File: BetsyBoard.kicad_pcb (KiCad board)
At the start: 2 copper layers, 50 x 50 mm, 44 parts, among them CON1 SDMMC_Card, P1 USB_OTG, P2 Analog, P3 Digital, P4 JLINK-SWD, P5 POWER, P6 CORTEX-JTAG, SW1 SW_PUSH, U1 STM32L486Rx-LQFP64, U2 TPS63051, U3 APX823, U4 PUSBM5V5X4, X1 XTAL, Y1 Crystal

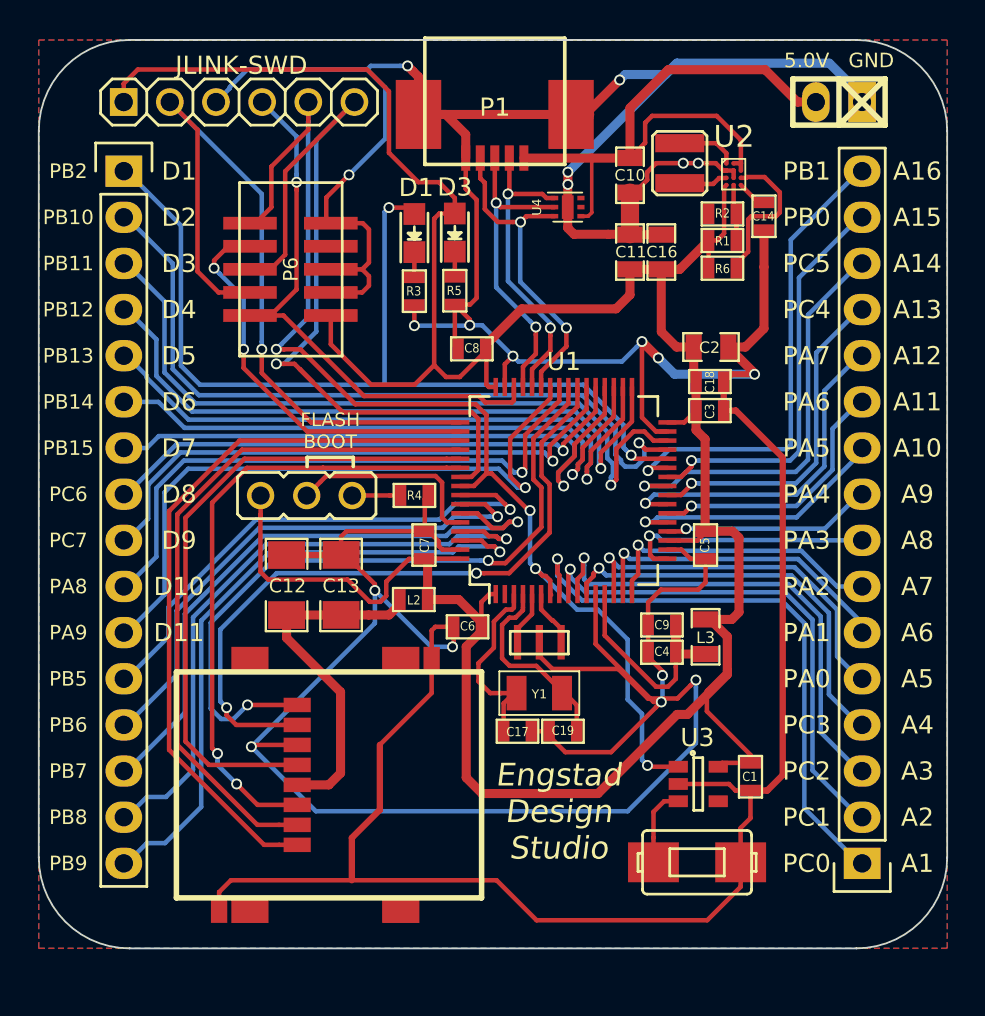
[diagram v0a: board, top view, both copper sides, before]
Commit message: Latest
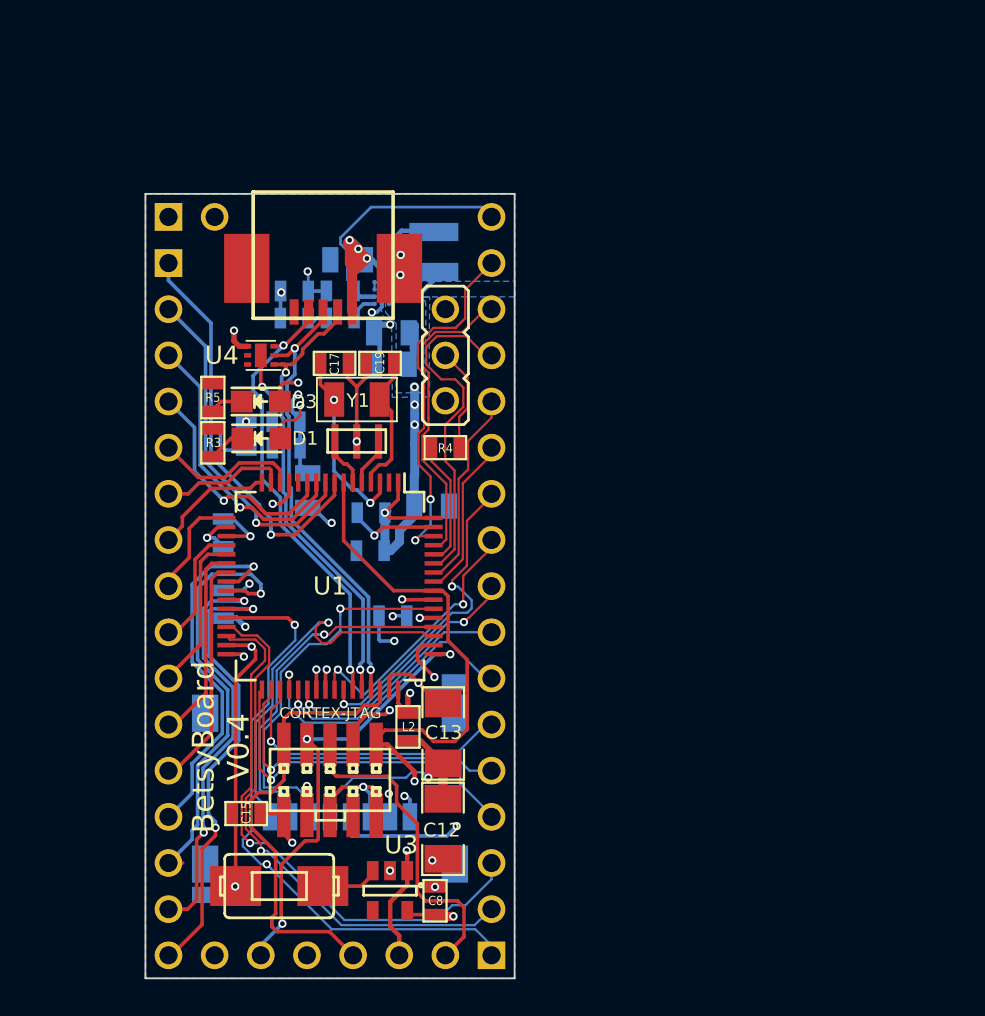
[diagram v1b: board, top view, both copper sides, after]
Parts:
- added ?: , xess:oshw-logo2, B.Cu at (112.5, 68.0)
- added C15: 0.1uF, smd:SM0603, F.Cu at (111.4, 92.6)
- added G***: LOGO, w_logo:Logo_silk_CC-BY-SA_5x2mm, B.Cu at (114.4, 79.8)
- added P7: PG, engstad:hdr-1x1, B.Cu at (124.9, 59.7)
- C1, C10, C11, C14, C16, C18, C2, C3, C4, C5, C6, C7, C9, CON1, L1, L3, R1, R2, R6, U2: moved to B.Cu
- L2: value 470nH -> 0.47uH
- P2, P3: footprint Pin_Headers:Pin_Header_Straight_1x16 -> engstad:pin-strip-16; moved to B.Cu
- P4: footprint xess:HDR_1x6 -> engstad:pin-strip-6; moved to B.Cu
- P5: footprint w_pin_strip:pin_socket_2 -> engstad:pin-socket-2
- P6: footprint engstad:smt-pin-header-02x05-127 -> engstad:conn-jtag-0.05
- moved P4 47.2 mm to (116.0, 100.4)
- moved P2 40.7 mm to (107.1, 81.3), turned to 270 degrees
- moved P5 36.2 mm to (108.4, 59.7), turned to 0 degrees
- moved P3 31.5 mm to (124.9, 81.3), turned to 90 degrees
- moved C1 30.5 mm to (110.2, 81.1), turned to 90 degrees
- moved C8 30.4 mm to (121.8, 97.4), turned to 90 degrees
- moved P6 28.2 mm to (116.0, 90.7), turned to 0 degrees
- moved C5 26.6 mm to (110.2, 77.1)
- moved C4 24.3 mm to (113.6, 71.0)
- moved R2 24.3 mm to (114.1, 65.3), turned to 0 degrees
- moved C14 24.0 mm to (116.6, 65.3), turned to 180 degrees
- moved R1 23.7 mm to (114.1, 63.8), turned to 180 degrees
- moved L3 23.3 mm to (114.8, 74.8), turned to 90 degrees
- moved SW1 23.0 mm to (113.2, 96.6), turned to 0 degrees
- moved C9 22.9 mm to (113.6, 72.5)
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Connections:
- net Net-(C12-Pad1) renamed /VDD_SD
- net Net-(R1-Pad2) renamed /FB
- JP1 pad 1: Net-(JP1-Pad1) -> GND
- JP1 pad 2: /BOOT0 -> Net-(JP1-Pad2)
- P5 pad 1: GND -> /OTG_5V
- P5 pad 2: /OTG_5V -> GND
- R4 pad 1: Net-(JP1-Pad1) -> /BOOT0
- R4 pad 2: GND -> Net-(JP1-Pad2)
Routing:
- net GND: track 338.3 -> 67.9 mm, vias 19 -> 17
- net VDD: track 163.1 -> 86.3 mm, vias 0 -> 15
- net /SDMMC_D1: track 39.2 -> 11.3 mm
- net /SDMMC_D0: track 38.3 -> 10.9 mm
- net /~RST: track 64.5 -> 38.8 mm, vias 4 -> 2
- net /D12: track 29.4 -> 8.91 mm, vias 1 -> 0
- net /SDMMC_D3: track 38.2 -> 19.3 mm, vias 0 -> 1
- net /D13: track 29.7 -> 11.0 mm, vias 1 -> 0
- net /SDMMC_D2: track 40.0 -> 21.3 mm, vias 0 -> 1
- net /D11: track 36.5 -> 17.9 mm, vias 1 -> 2
- net /D5: track 35.9 -> 17.5 mm
- net /D15: track 35.2 -> 17.0 mm, vias 1 -> 0
- net /D10: track 32.8 -> 14.9 mm, vias 1 -> 2
- net /D7: track 34.7 -> 16.8 mm
- net /D6: track 34.0 -> 16.2 mm
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- added copper zone on In2.Cu, net /OTG_5V
- added copper zone on In1.Cu, net GND
- added copper zone on In2.Cu, net GND
- added copper zone on B.Cu, net VDD
- added copper zone on In2.Cu, net VDD
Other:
- board size 50 x 50 mm -> 20.3 x 43.2 mm
- copper layers 2 -> 4
- net class Default: clearance 0.2 -> 0.1
- rule trace_clearance: 0.2 -> 0.1
- rule via_min_drill: 0.3 -> 0.254
- rule via_min_size: 0.4 -> 0.4572
- board text added: "+"
- board text added: "10"
- board text added: "11"
- board text added: "12"
- board text added: "13"
- board text added: "14"
- board text added: "15"
- board text added: "16"
- board text added: "3"
- board text added: "6"
- board text added: "7"
- board text added: "BetsyBoard V0.4"
- board text added: "No warranty! Use or reproduce at your own risk!"
- board text added: "PG"
- board text added: "SWO ~RST~ SWD GND CLK VDD"
- board text removed: "5.0V"
- board text removed: "A10"
- board text removed: "A11"
- board text removed: "A12"
- board text removed: "A13"
- board text removed: "A14"
- board text removed: "A15"
- board text removed: "A16"
- board text removed: "A7"
- board text removed: "D11"
- board text removed: "D3"
- board text removed: "D6"
- board text removed: "FLASH BOOT"
- board text removed: "GND"
- board text removed: "PA0"
- board text removed: "PA1"
- board text removed: "PA2"
- board text removed: "PA3"
- board text removed: "PA4"
- board text removed: "PA5"
- board text removed: "PA6"
- board text removed: "PA7"
- board text removed: "PA8"
- board text removed: "PA9"
- board text removed: "PB0"
- board text removed: "PB1"
- board text removed: "PB10"
- board text removed: "PB11"
- board text removed: "PB12"
- board text removed: "PB13"
- board text removed: "PB14"
- board text removed: "PB15"
- board text removed: "PB2"
- board text removed: "PB5"
- board text removed: "PB6"
- board text removed: "PB7"
- board text removed: "PB8"
- board text removed: "PB9"
- board text removed: "PC0"
- board text removed: "PC1"
- board text removed: "PC2"
- board text removed: "PC3"
- board text removed: "PC4"
- board text removed: "PC5"
- board text removed: "PC6"
- board text removed: "PC7"
